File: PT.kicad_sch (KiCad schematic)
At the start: 4 parts

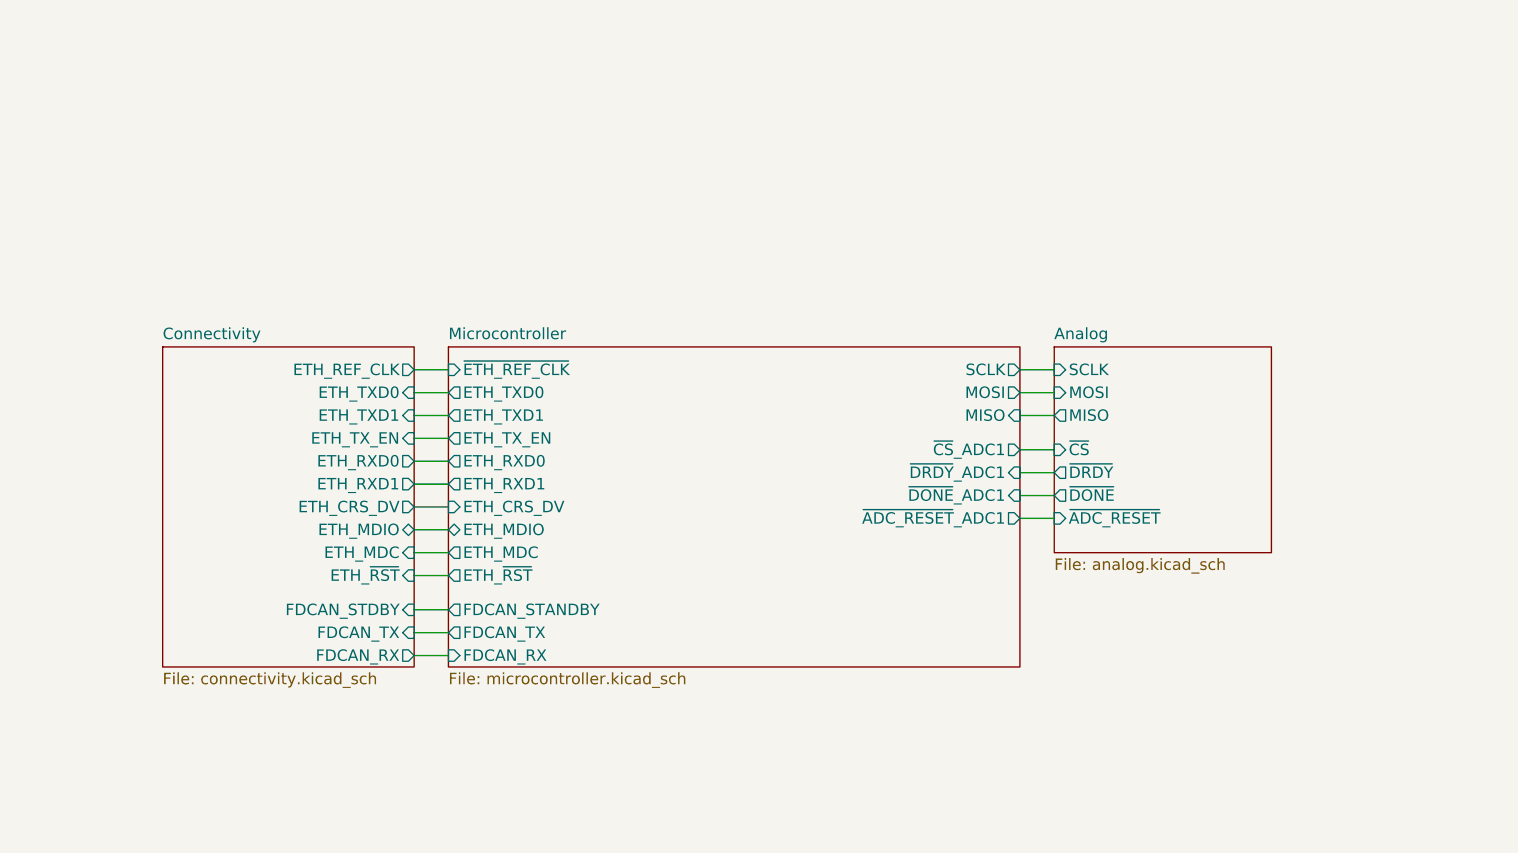
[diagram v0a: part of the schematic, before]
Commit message: holy hell 2 adcs
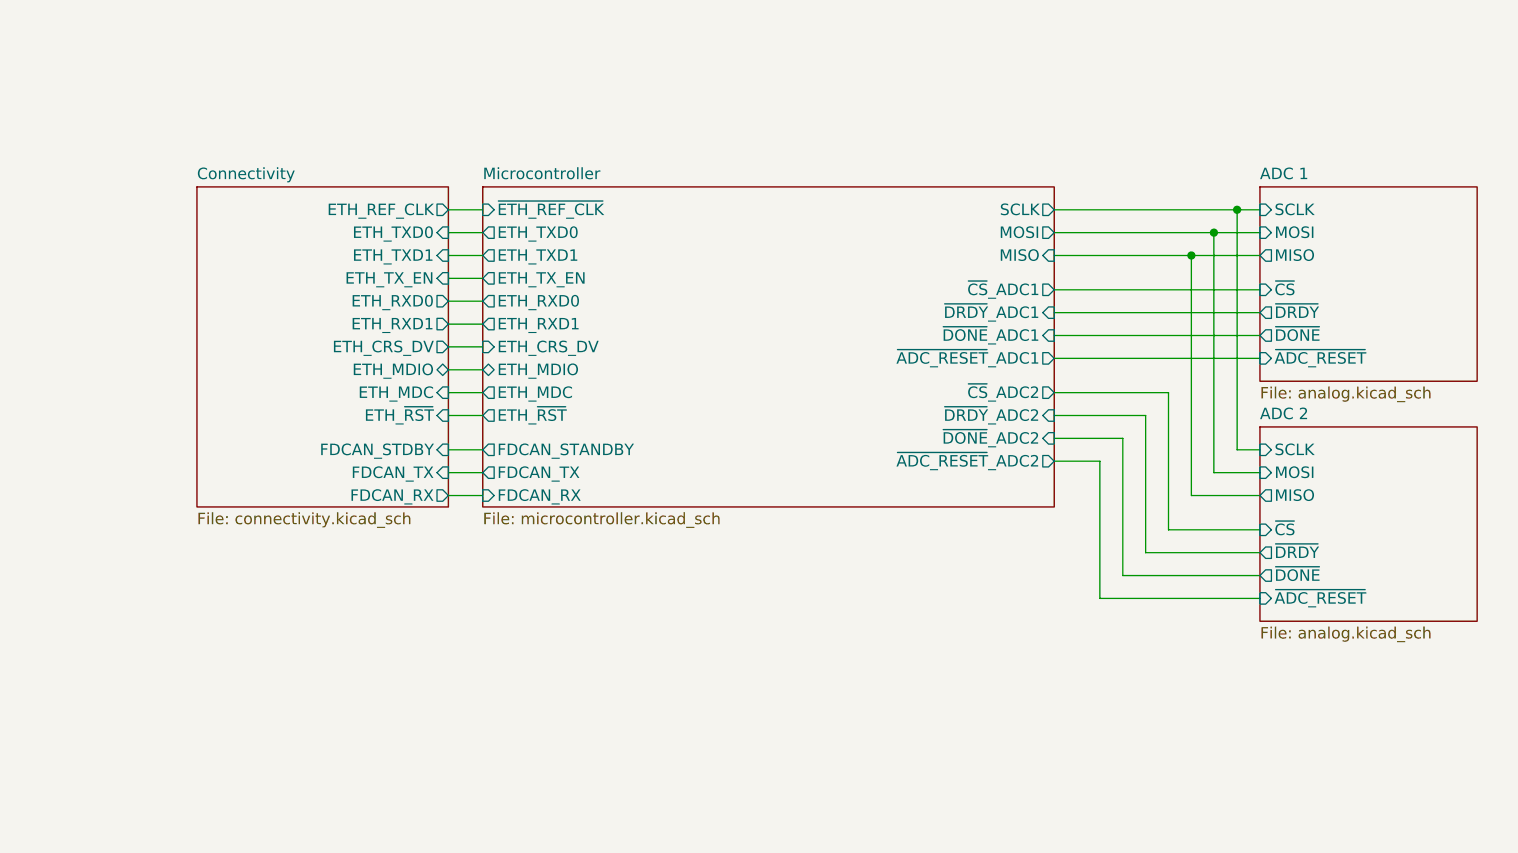
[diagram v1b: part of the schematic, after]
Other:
- sheet Analog renamed ADC 1
- added sheet ADC 2 (analog.kicad_sch)
- sheet Microcontroller ports: added ~{ADC_RESET}_ADC2, ~{CS}_ADC2, ~{DONE}_ADC2, ~{DRDY}_ADC2; removed none
